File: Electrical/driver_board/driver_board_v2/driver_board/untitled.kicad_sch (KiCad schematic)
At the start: 17 parts, among them J1 Conn_01x04_Pin, SW1 SW_Nidec_CAS-120A1, U1 STM32F446RETx, Y1 8Mhz

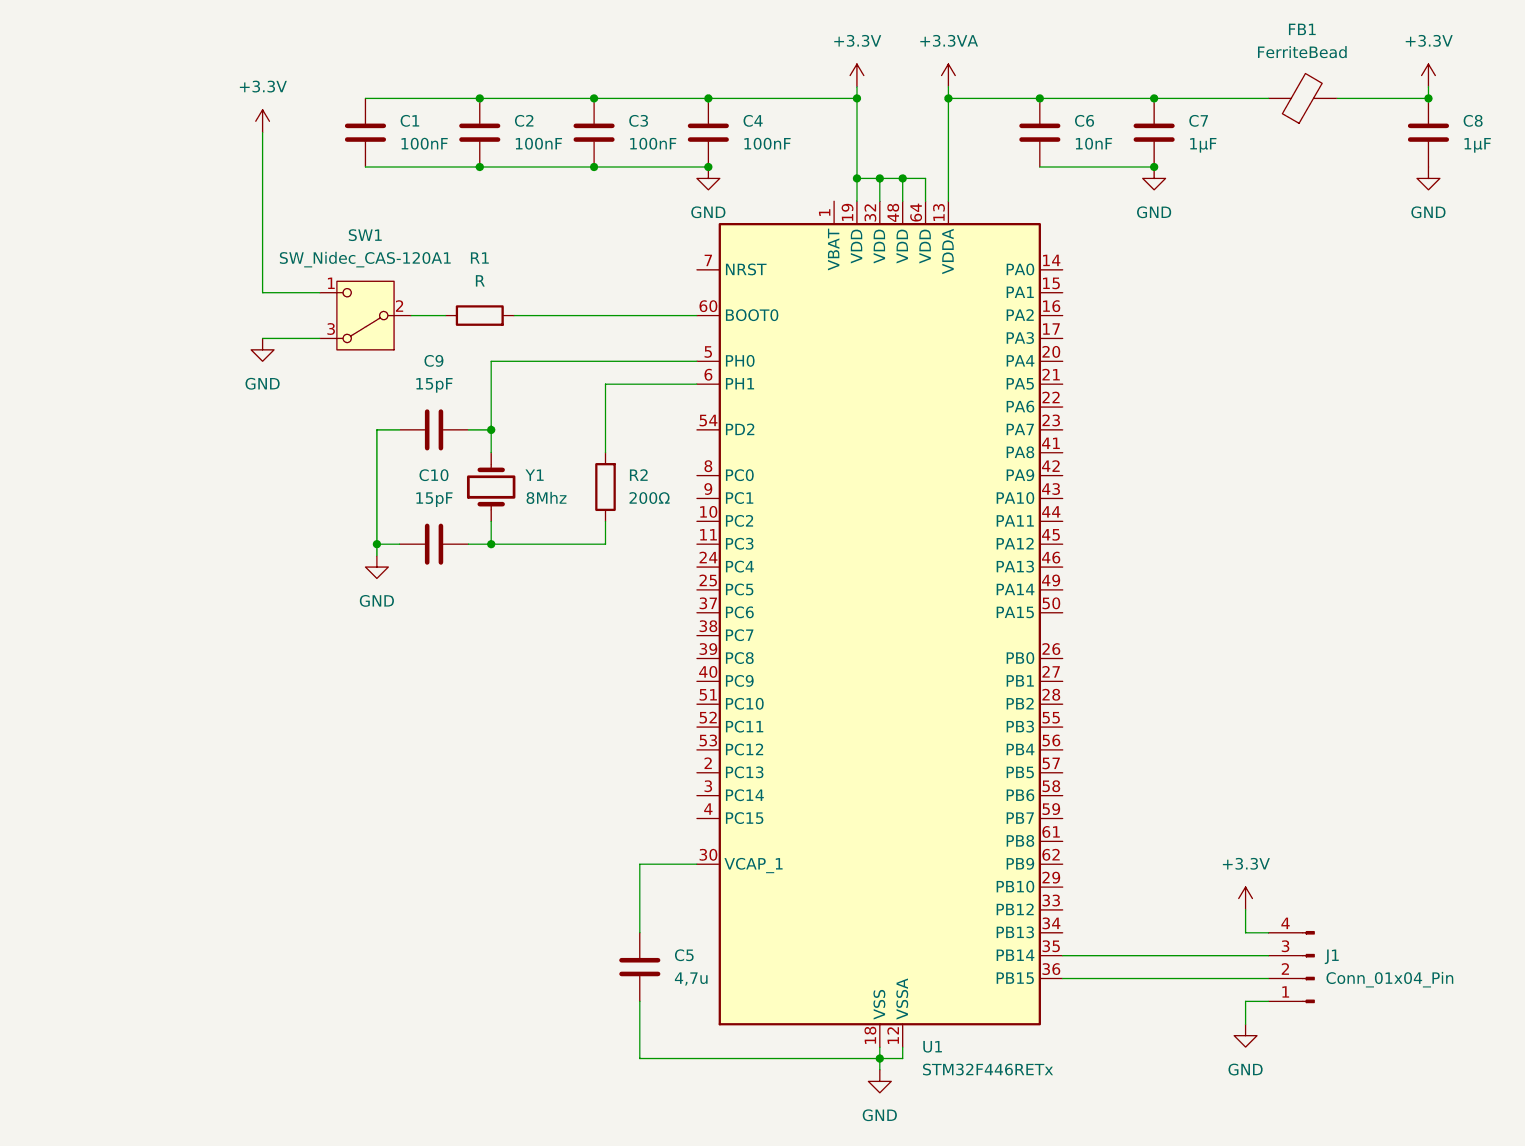
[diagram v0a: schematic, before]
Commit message: Updates to MCU
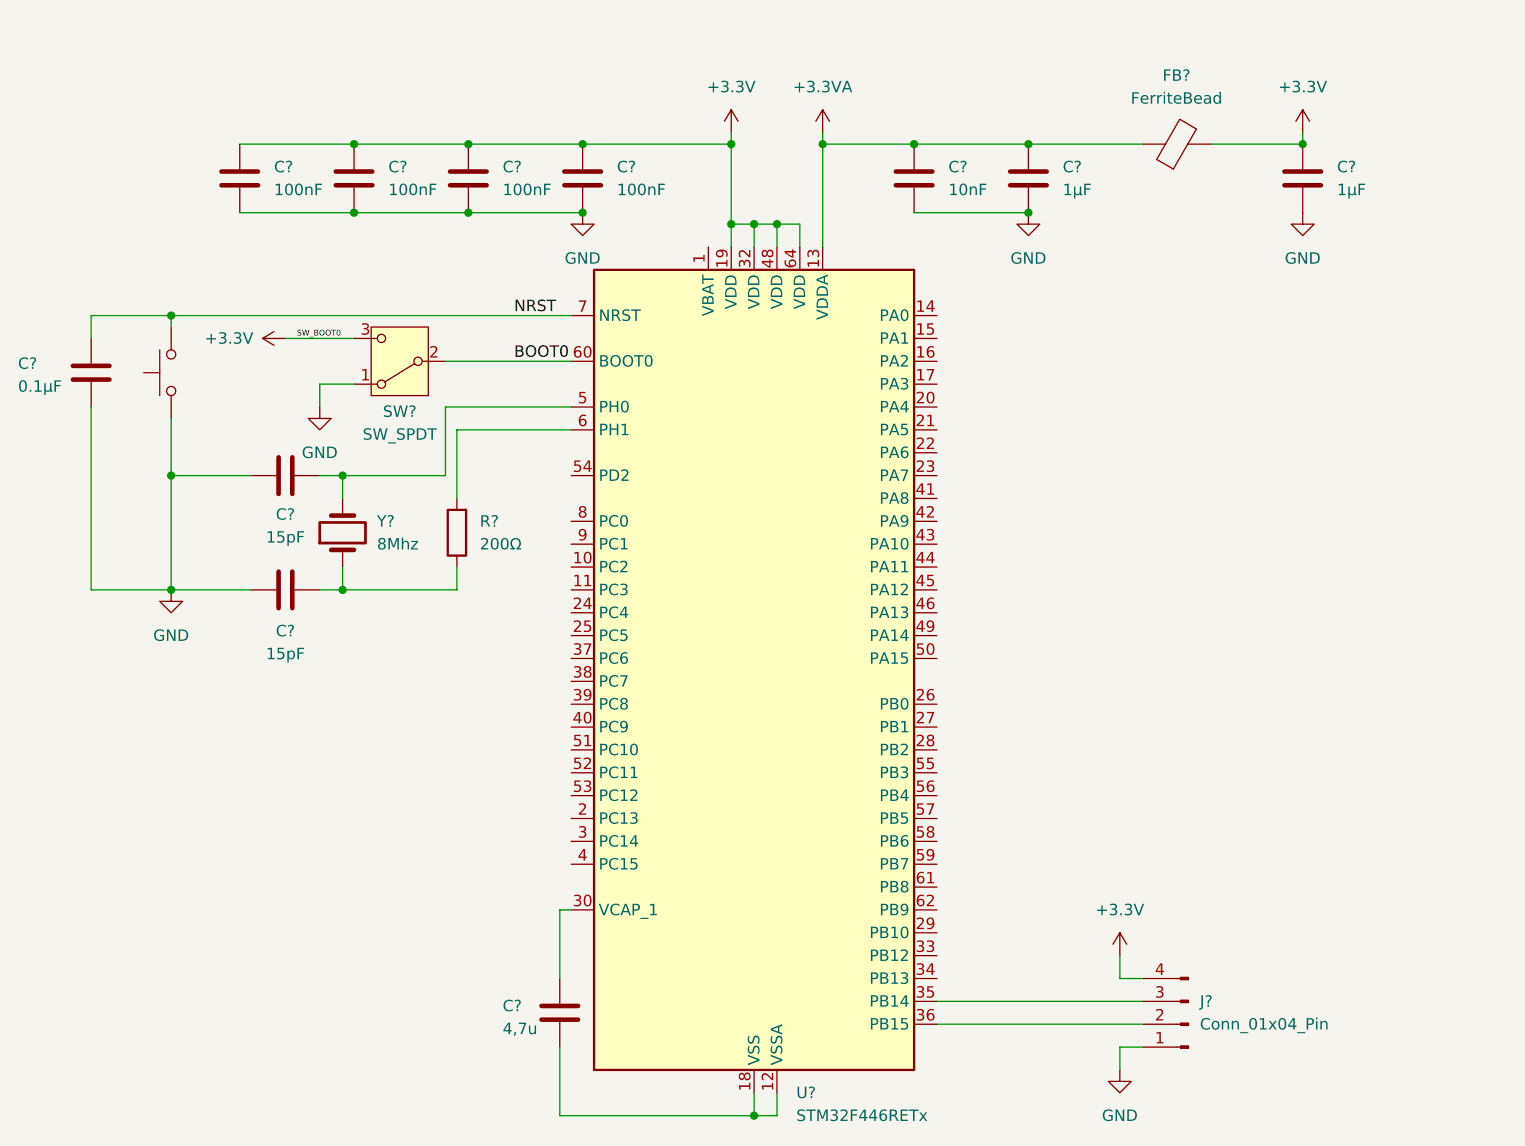
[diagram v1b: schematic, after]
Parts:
- removed C1, C2, C3, C4: 100nF, symbol Device:C
- removed C10, C9: 15pF, symbol Device:C
- removed C5: 4,7u, symbol Device:C
- removed C6: 10nF, symbol Device:C
- removed C7, C8: 1µF, symbol Device:C
- removed J1: Conn_01x04_Pin, symbol Connector:Conn_01x04_Pin
- removed R1: R, symbol Device:R
- removed R2: 200Ω, symbol Device:R
- removed SW1: SW_Nidec_CAS-120A1, Button_Switch_SMD:Nidec_Copal_CAS-120A, symbol Switch:SW_Nidec_CAS-120A1
- removed U1: STM32F446RETx, Package_QFP:LQFP-64_10x10mm_P0.5mm, symbol MCU_ST_STM32F4:STM32F446RETx
- removed Y1: 8Mhz, symbol Device:Crystal
- added C? (x2): 15pF, symbol Device:C
- added C? (x4): 100nF, symbol Device:C
- added C? (x2): 1µF, symbol Device:C
- added C?: 0.1µF, symbol Device:C
- added C?: 4,7u, symbol Device:C
- added C?: 10nF, symbol Device:C
- added J?: Conn_01x04_Pin, symbol Connector:Conn_01x04_Pin
- added R?: 200Ω, symbol Device:R
- added SW?: SW_Push, symbol Switch:SW_Push
- added SW?: SW_SPDT, symbol Switch:SW_SPDT
- added U?: STM32F446RETx, Package_QFP:LQFP-64_10x10mm_P0.5mm, symbol MCU_ST_STM32F4:STM32F446RETx
- added Y?: 8Mhz, symbol Device:Crystal
- renumbered FB1 to FB?
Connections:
- net +3.3V: now also C?.1, C?.1, C?.1, C?.1, C?.1, J?.4 (Pin_4), SW?.3 (C), U?.19 (VDD), U?.32 (VDD), U?.48 (VDD), U?.64 (VDD)
- net +3.3VA: now also C?.1, C?.1, U?.13 (VDDA)
- net GND: now also C?.1, C?.1, C?.1, C?.2, C?.2, C?.2, C?.2, C?.2, C?.2, C?.2, J?.1 (Pin_1), SW?.1, SW?.1 (A)
- new net: C?.2, U?.5 (PH0), Y?.2
- new net: C?.2, R?.1, Y?.1
- new net: R?.2, U?.6 (PH1)
- new net: C?.1, U?.12 (VSSA), U?.18 (VSS), U?.31 (VSS), U?.47 (VSS), U?.63 (VSS)
- new net: C?.2, U?.30 (VCAP_1)
- new net: J?.3 (Pin_3), U?.35 (PB14)
- new net: J?.2 (Pin_2), U?.36 (PB15)
- new net BOOT0: SW?.2 (B), U?.60 (BOOT0)
- new net NRST: C?.2, SW?.2, U?.7 (NRST)
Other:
- moved on the sheet: FB?
